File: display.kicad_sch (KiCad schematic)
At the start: 215 parts, among them U31 74HC595, U32 74HC595, U33 ULN2003, U34 ULN2003, U35 4028

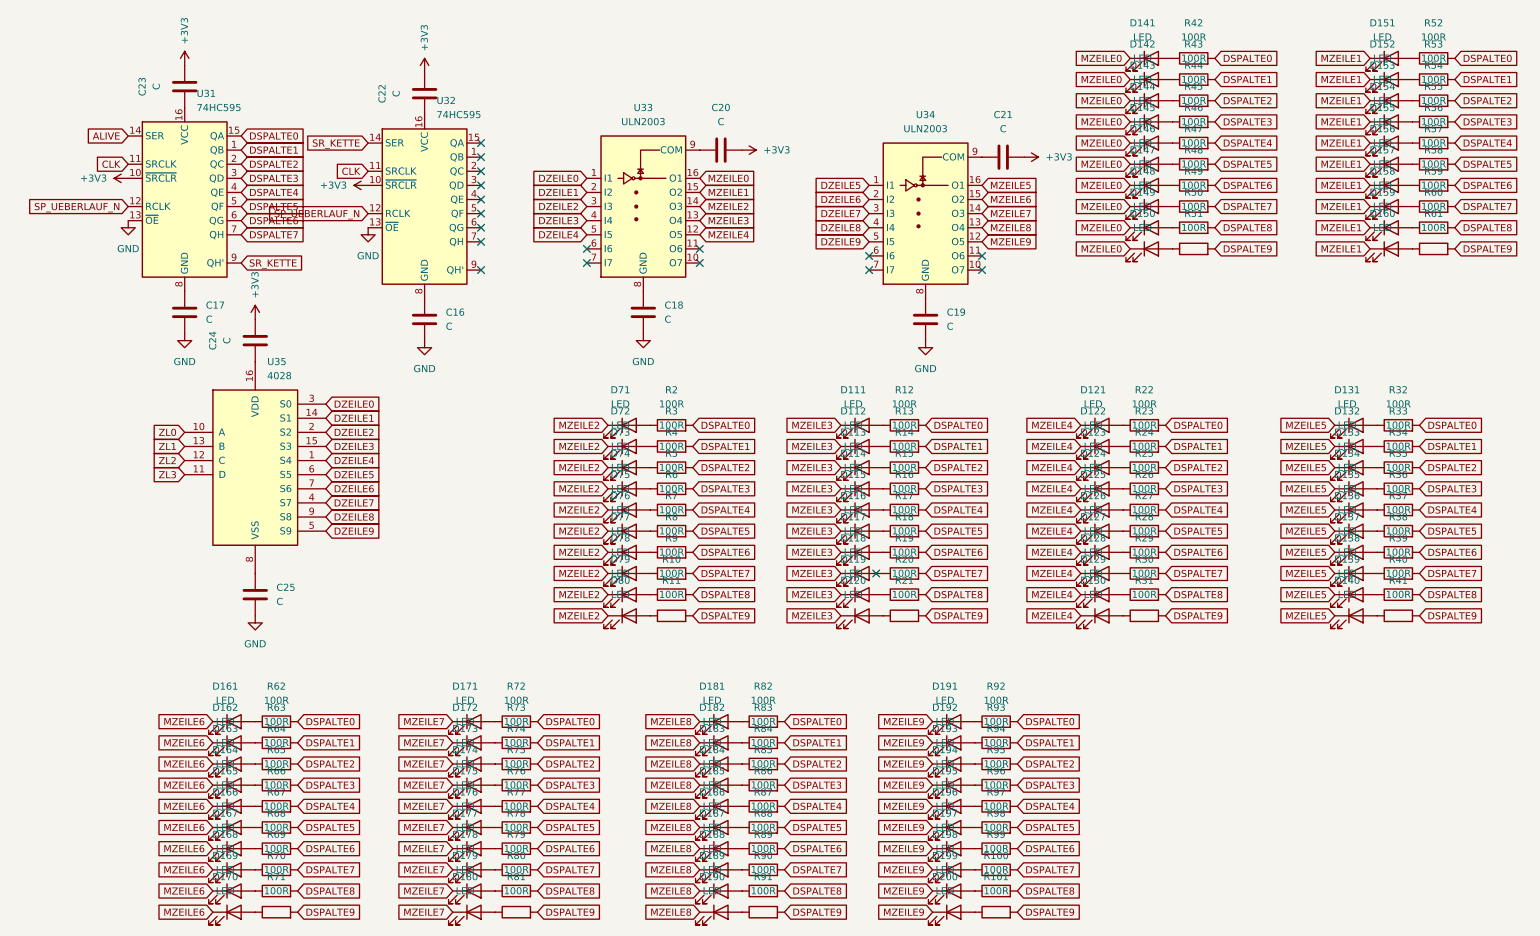
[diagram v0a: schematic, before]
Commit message: very big comit what i did is in the description
jooo so this is what i did i fixed all erc errors now it is basicly finished and also started to make a website where you can lern how this whole thing works and also have a simulation for it but it is still in progress so right now chapter 1 is complete with all the simulations and right now i am working on chapter 6 it should not take very long untill i am finished i will probaply post more comits in the future so yea sry that i forgot to do that ig
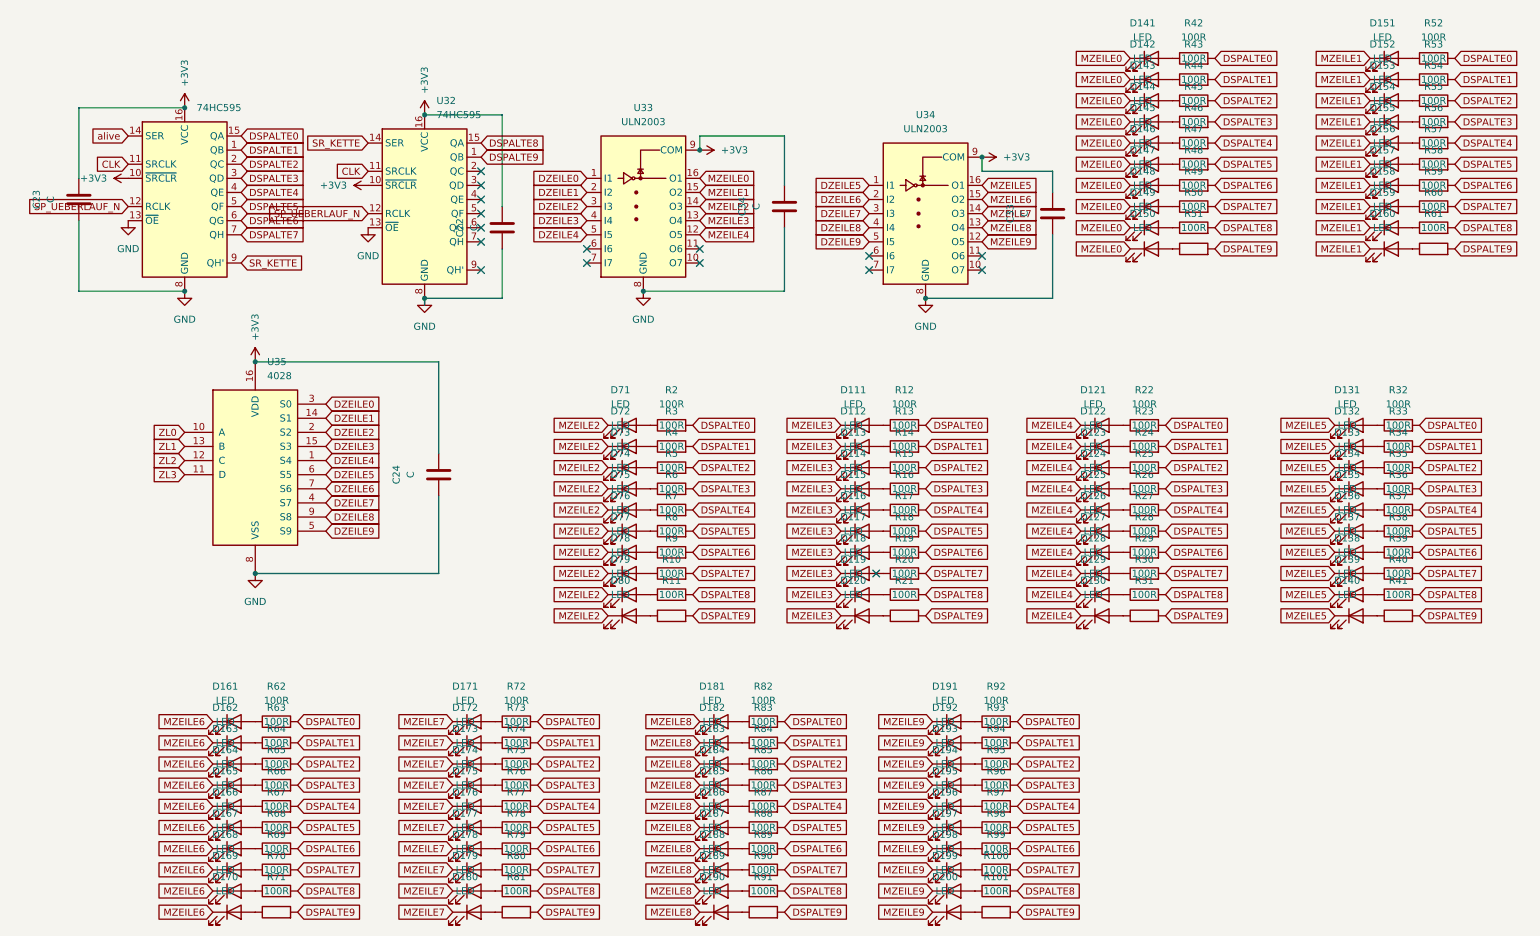
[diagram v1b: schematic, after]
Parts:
- removed C16, C17, C18, C19, C20, C21, C25: C, symbol Device:C
- added C33, C34: C, symbol Device:C
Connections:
- net +3V3: now also U31.16 (VCC), U32.16 (VCC), U33.9 (COM), U34.9 (COM), U35.16 (VDD), C33.1, C34.1
- net DSPALTE8: now also U32.15 (QA)
- net DSPALTE9: now also U32.1 (QB)
- net GND: now also C22.2, C23.2, C24.2, U31.8 (GND), U32.8 (GND), U33.8 (GND), U34.8 (GND), U35.8 (VSS), C33.2, C34.2
- net ALIVE renamed alive
- no-connect marks 18 -> 16
